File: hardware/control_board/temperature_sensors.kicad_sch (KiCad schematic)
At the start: 23 parts, among them J5 RTD, J5 TC, U2 MAX6675, U6 MCP6N11T-005E, U7 MCP6001T

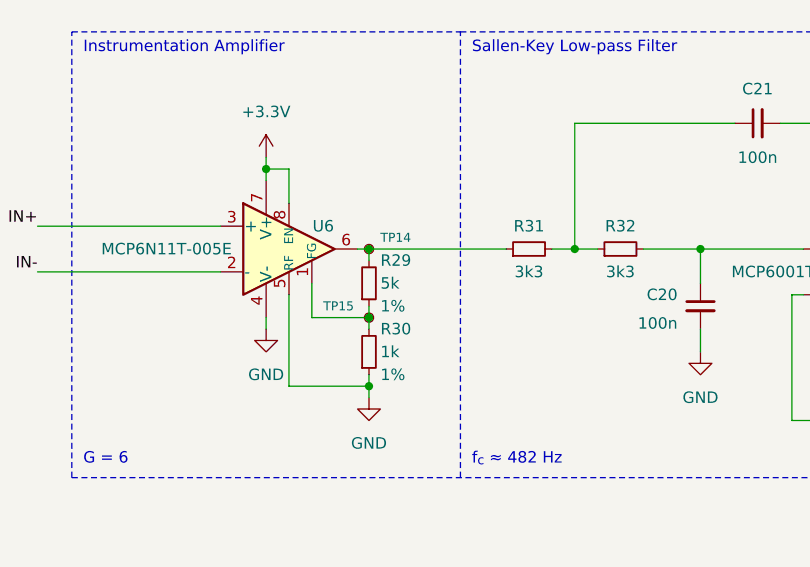
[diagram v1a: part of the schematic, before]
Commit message: Cleanup the project
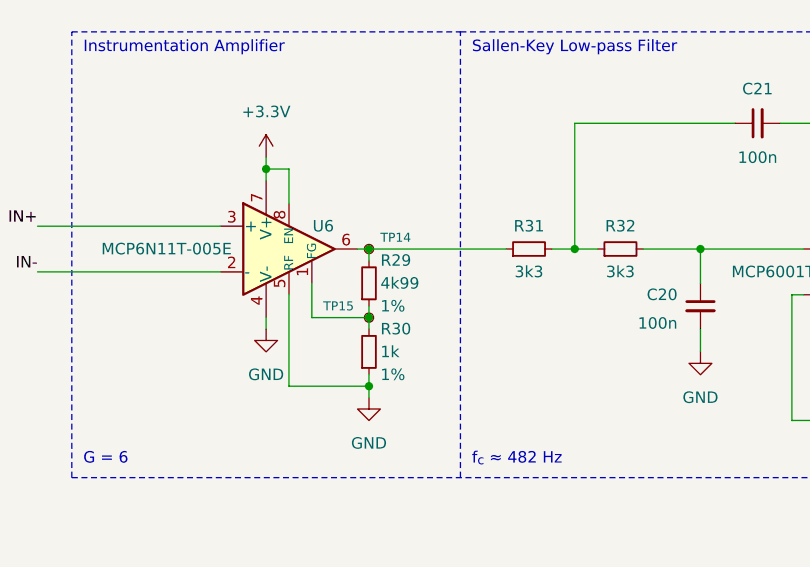
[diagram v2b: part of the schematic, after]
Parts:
- R29: value 5k -> 4k99
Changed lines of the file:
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@@
       (effects (font (size 1.27 1.27)) (justify left))
     )
-    (property "Value" "5k" (at 147.32 62.23 0)
+    (property "Value" "4k99" (at 147.32 62.23 0)
       (effects (font (size 1.27 1.27)) (justify left))
     )
